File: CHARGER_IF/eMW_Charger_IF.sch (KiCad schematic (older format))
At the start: 13 parts, among them J1 CONN_01X02, J2 Booster_J1_J3, J3 Booster_J4_J2, U1 V7805-2000R, U2 ArduinoSocket, U3 SN74ACT08N, U4 SN74ACT08N

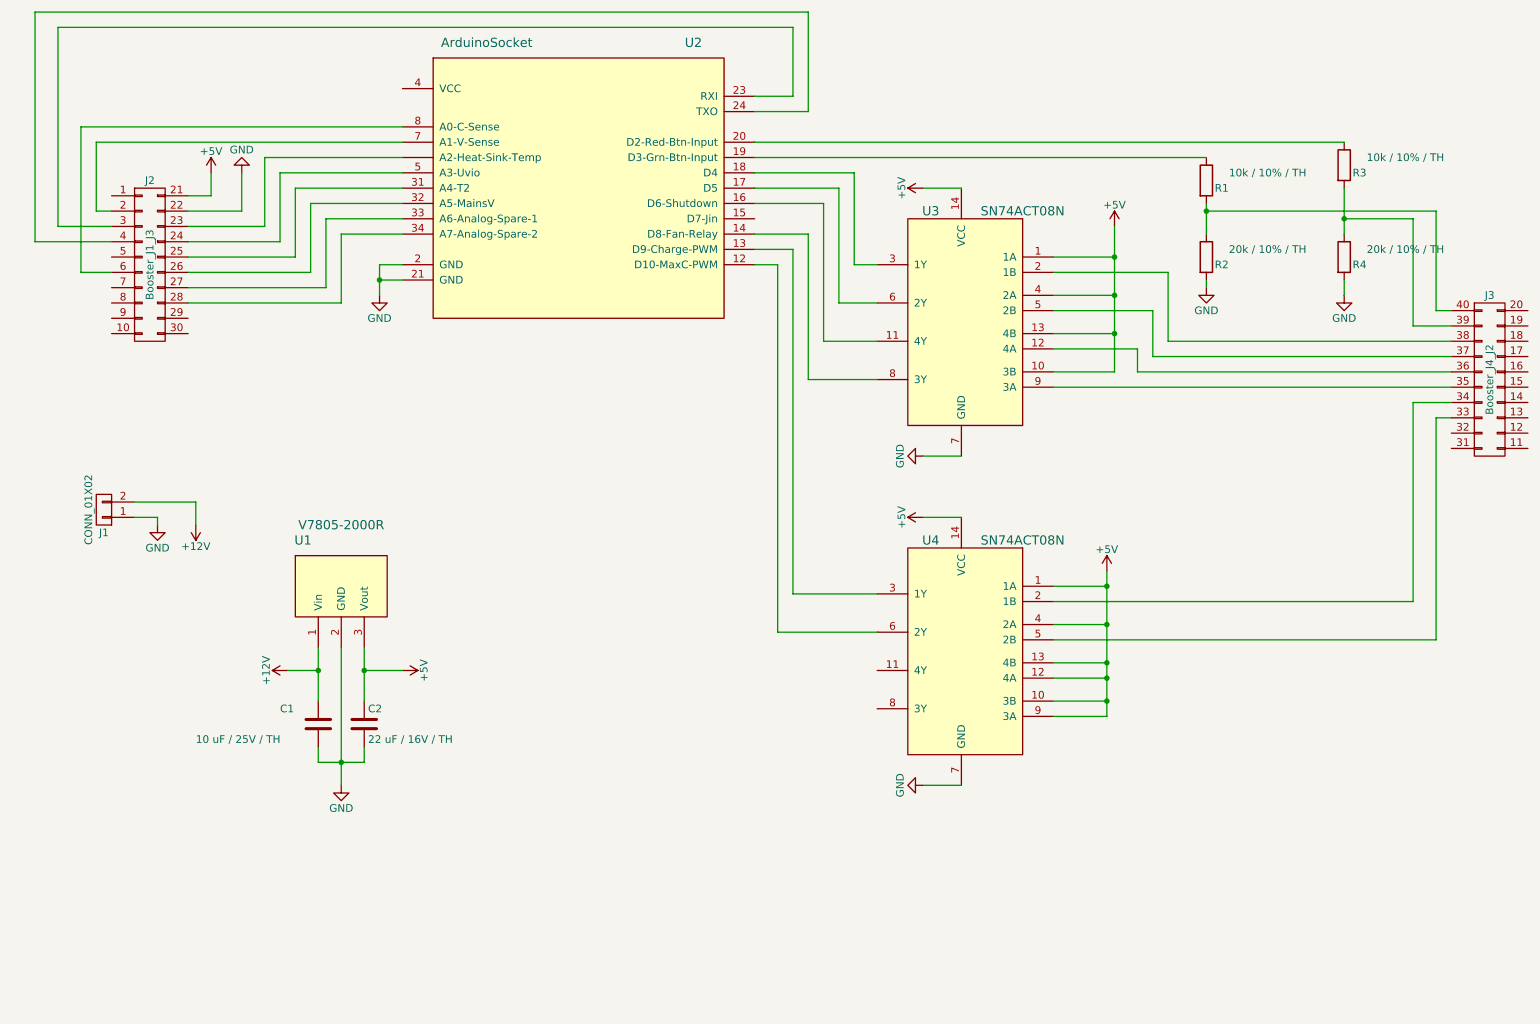
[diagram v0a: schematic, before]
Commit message: Charger IF WIP
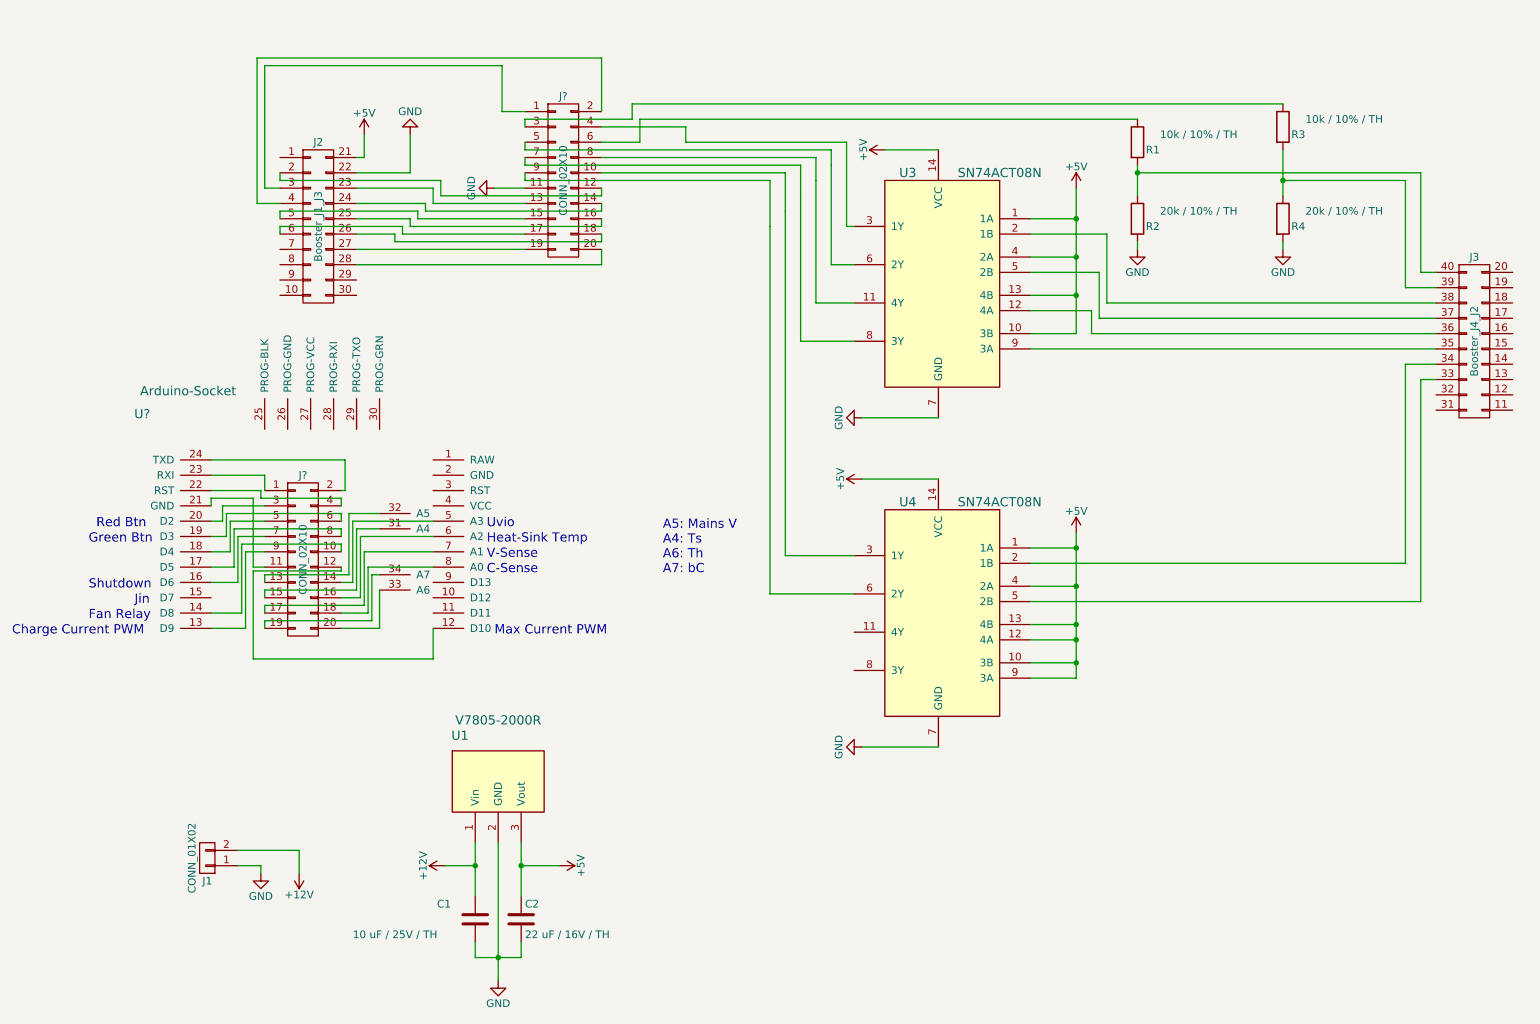
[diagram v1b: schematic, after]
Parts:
- removed U2: ArduinoSocket, Pin_Headers:Pin_Header_Straight_2x10_Pitch2.54mm, symbol ArduinoSocket
- added J? (x2): CONN_02X10, symbol CONN_02X10
- added U?: Arduino-Socket, symbol Arduino-Socket
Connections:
- net GND: now also J?.11 (P11)
- net at U4.6 (2Y): now also J?.9 (P9)
- net at U4.3 (1Y): now also J?.10 (P10)
- net at U3.8 (3Y): now also J?.7 (P7)
- net at U3.11 (4Y): now also J?.8 (P8)
- net at U3.6 (2Y): now also J?.5 (P5)
- net at U3.3 (1Y): now also J?.4 (P4)
- net at R1.1: now also J?.6 (P6)
- net at R3.1: now also J?.3 (P3)
- net at J2.3 (P3): now also J?.1 (P1)
- net at J2.4 (P4): now also J?.2 (P2)
- net at J2.25 (P25): now also J?.16 (P16)
- net at J2.26 (P26): now also J?.18 (P18)
- net at J2.27 (P27): now also J?.19 (P19)
- net at J2.28 (P28): now also J?.20 (P20)
- net at J2.24 (P24): now also J?.14 (P14)
- net at J2.2 (P2): now also J?.12 (P12)
- net at J2.6 (P6): now also J?.17 (P17)
- net at J2.23 (P23): now also J?.13 (P13)
- net at J2.5 (P5): now also J?.15 (P15)
- new net: J?.12 (P12), U?.12 (D10)
- new net: J?.9 (P9), U?.13 (D9)
- new net: J?.10 (P10), U?.14 (D8)
- new net: J?.7 (P7), U?.16 (D6)
- new net: J?.8 (P8), U?.17 (D5)
- new net: J?.5 (P5), U?.18 (D4)
- new net: J?.6 (P6), U?.19 (D3)
- new net: J?.3 (P3), U?.20 (D2)
- new net: J?.11 (P11), U?.21 (GND)
- new net: J?.4 (P4), U?.22 (RST)
- new net: J?.1 (P1), U?.23 (RXI)
- new net: J?.2 (P2), U?.24 (TXD)
- new net: J?.15 (P15), U?.31 (A4)
- new net: J?.13 (P13), U?.32 (A5)
- new net: J?.20 (P20), U?.33 (A6)
- new net: J?.19 (P19), U?.34 (A7)
- new net: J?.14 (P14), U?.5 (A3)
- new net: J?.16 (P16), U?.6 (A2)
- new net: J?.17 (P17), U?.7 (A1)
- new net: J?.18 (P18), U?.8 (A0)
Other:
- note added: "A5: Mains V\nA4: Ts\nA6: Th\nA7: bC"
- note added: "C-Sense"
- note added: "Charge Current PWM"
- note added: "Fan Relay"
- note added: "Green Btn"
- note added: "Heat-Sink Temp"
- note added: "Jin"
- note added: "Max Current PWM"
- note added: "Red Btn"
- note added: "Shutdown"
- note added: "Uvio"
- note added: "V-Sense"
- moved on the sheet: C1, C2, J1, J2, J3, R1, R2, R3, R4, U1, U3, U4
